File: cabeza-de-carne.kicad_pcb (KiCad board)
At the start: 2 copper layers, 25.7 x 29.8 mm, 20 parts, among them J1 Stomp_Connector, J2 Power_Connector, Q1 2N3904, Q2 BC182L

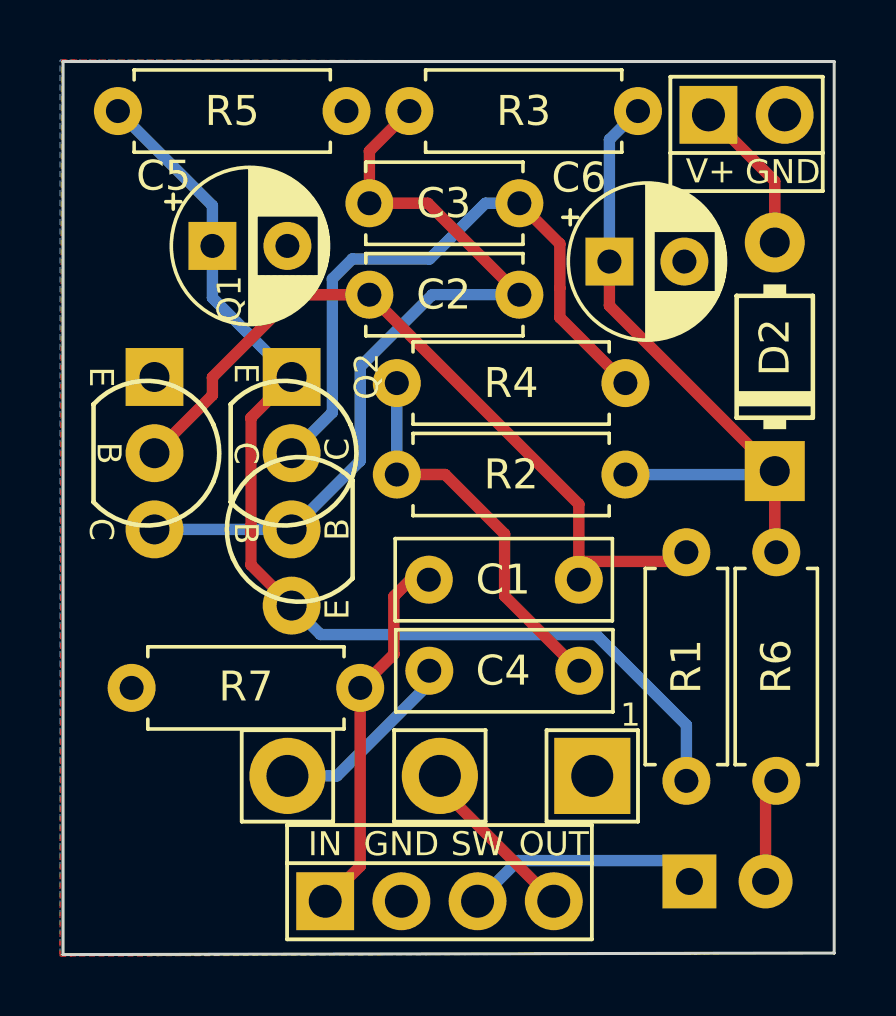
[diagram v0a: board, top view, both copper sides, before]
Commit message: v0.3 gerbers, images
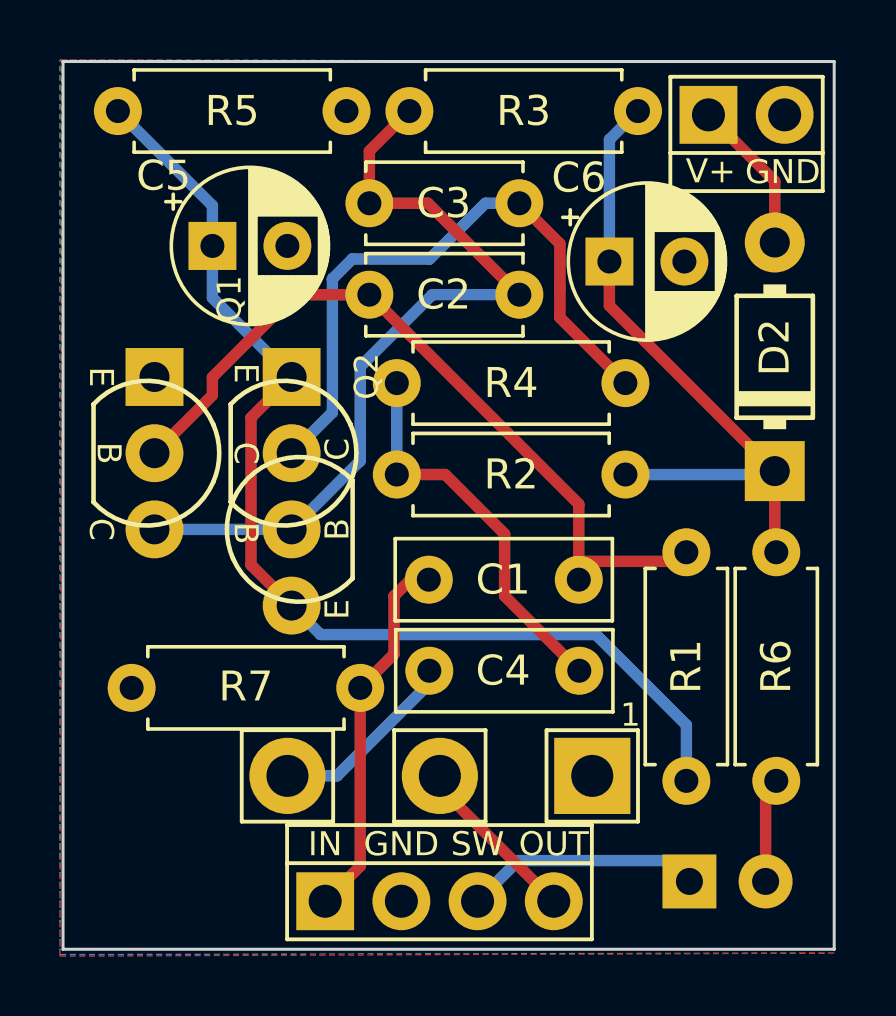
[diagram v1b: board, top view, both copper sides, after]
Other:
- board size 25.7 x 29.8 mm -> 25.7 x 29.6 mm
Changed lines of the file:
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@@
   (page "A4")
   (layers
-    (0 "F.Cu" signal)
-    (31 "B.Cu" signal)
+    (0 "F.Cu" signal hide)
+    (31 "B.Cu" signal hide)
     (32 "B.Adhes" user)
     (33 "F.Adhes" user)
@@
     (47 "F.CrtYd" user)
     (48 "B.Fab" user)
-    (49 "F.Fab" user)
+    (49 "F.Fab" user hide)
   )
   (setup
@@
       (dielectric_constraints no)
     )
-    (last_trace_width 0.381)
+    (last_trace_width 0.25)
     (user_trace_width 0.254)
     (user_trace_width 0.381)
@@
     (effects (font (size 1.1 0.95) (thickness 0.15)) (justify mirror))
   )
-  (gr_line (start 250.698 -54.102) (end 250.698 -24.384) (layer "Edge.Cuts") (width 0.1))
+  (gr_line (start 250.698 -54.102) (end 250.698 -24.511) (layer "Edge.Cuts") (width 0.1))
   (gr_line (start 224.9932 -54.102) (end 250.698 -54.102) (layer "Edge.Cuts") (width 0.1))
-  (gr_line (start 224.9932 -24.3332) (end 224.9932 -54.102) (layer "Edge.Cuts") (width 0.1))
-  (gr_line (start 250.698 -24.384) (end 224.9932 -24.3332) (layer "Edge.Cuts") (width 0.1))
+  (gr_line (start 224.9932 -24.511) (end 224.9932 -54.102) (layer "Edge.Cuts") (width 0.1))
+  (gr_line (start 250.698 -24.511) (end 224.9932 -24.511) (layer "Edge.Cuts") (width 0.1))
   (segment (start 232.473501 -30.289499) (end 234.124499 -30.289499) (width 0.381) (layer "B.Cu") (net 5))
   (segment (start 234.124499 -30.289499) (end 237.2017 -33.3667) (width 0.381) (layer "B.Cu") (net 5))
